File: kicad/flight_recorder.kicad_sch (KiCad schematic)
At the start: 12 parts, among them Q3 FS8205A, U1 ESP32-C3-SuperMini, U2 DW01A, U3 MCP1700x-330xxTT

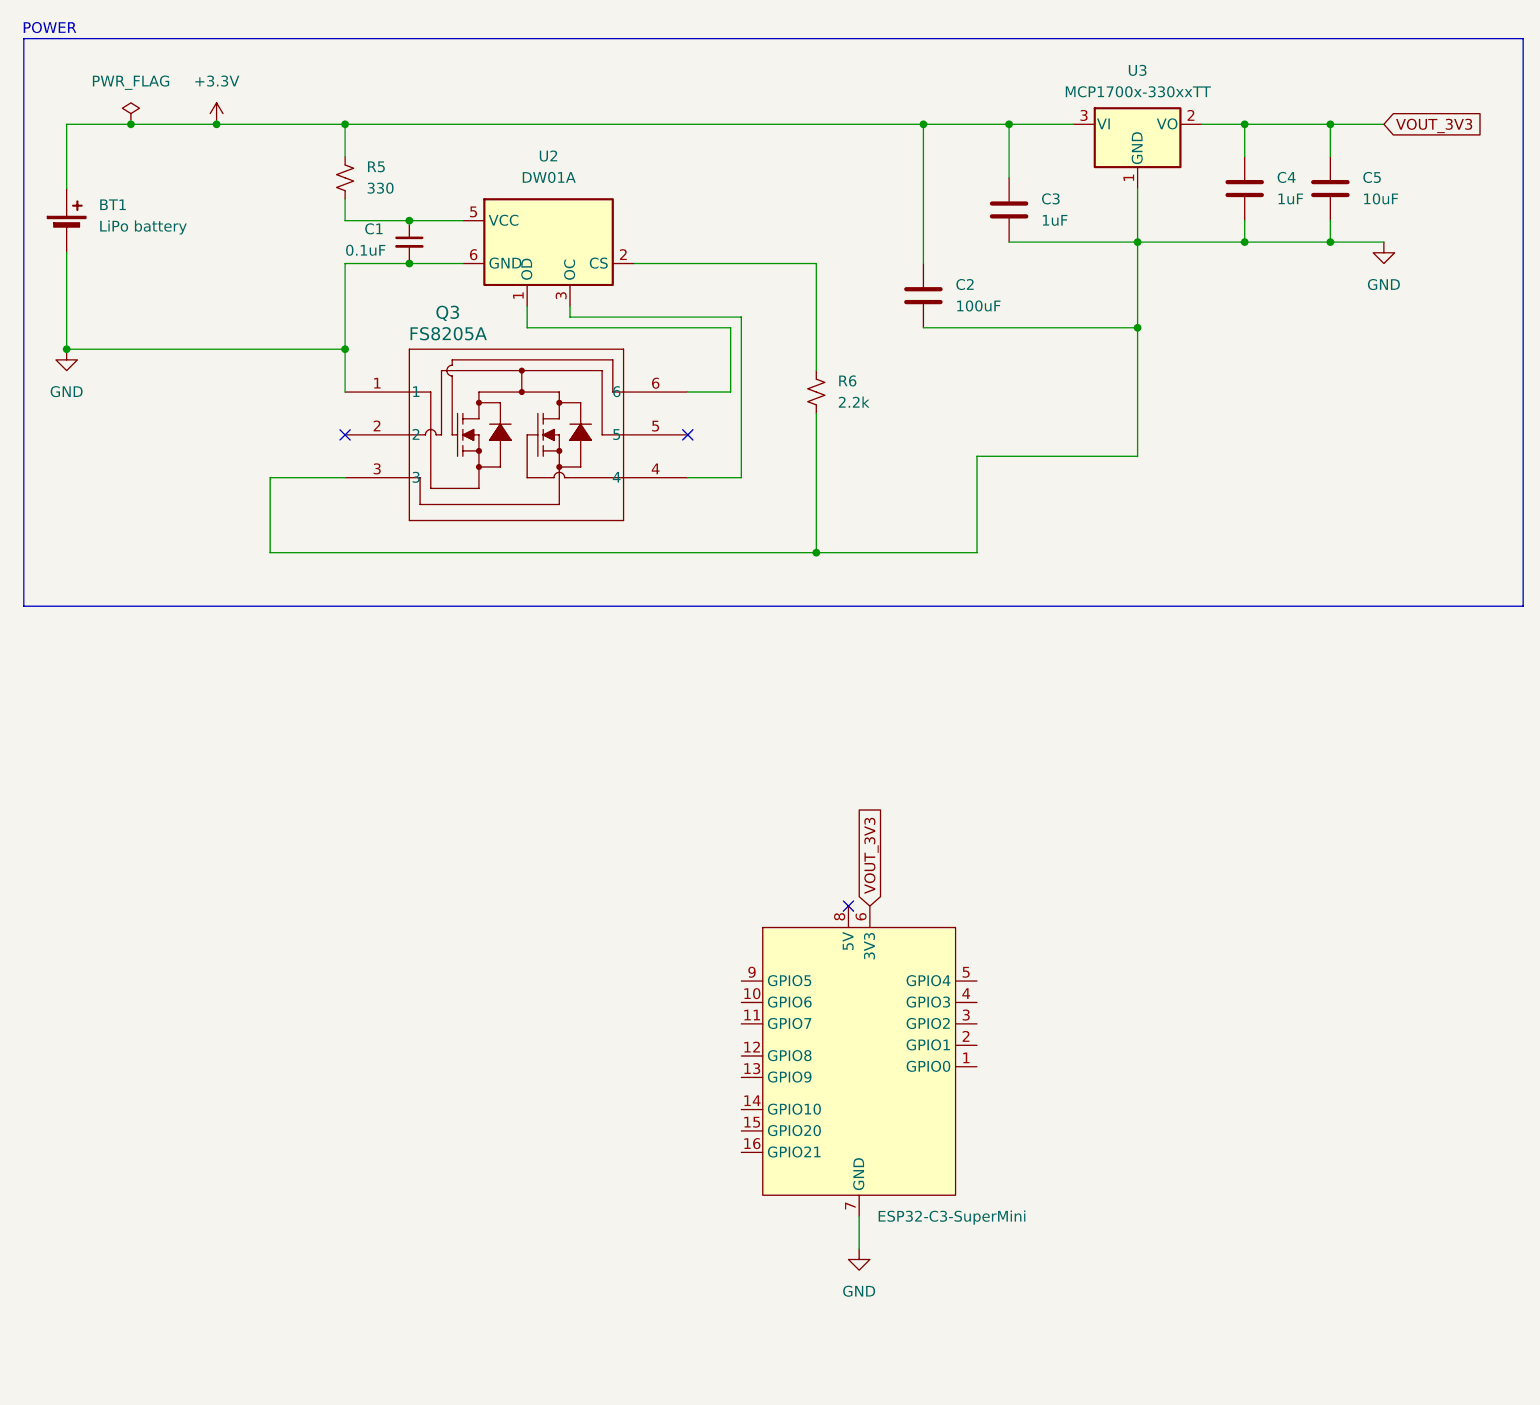
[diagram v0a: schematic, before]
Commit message: added sensors
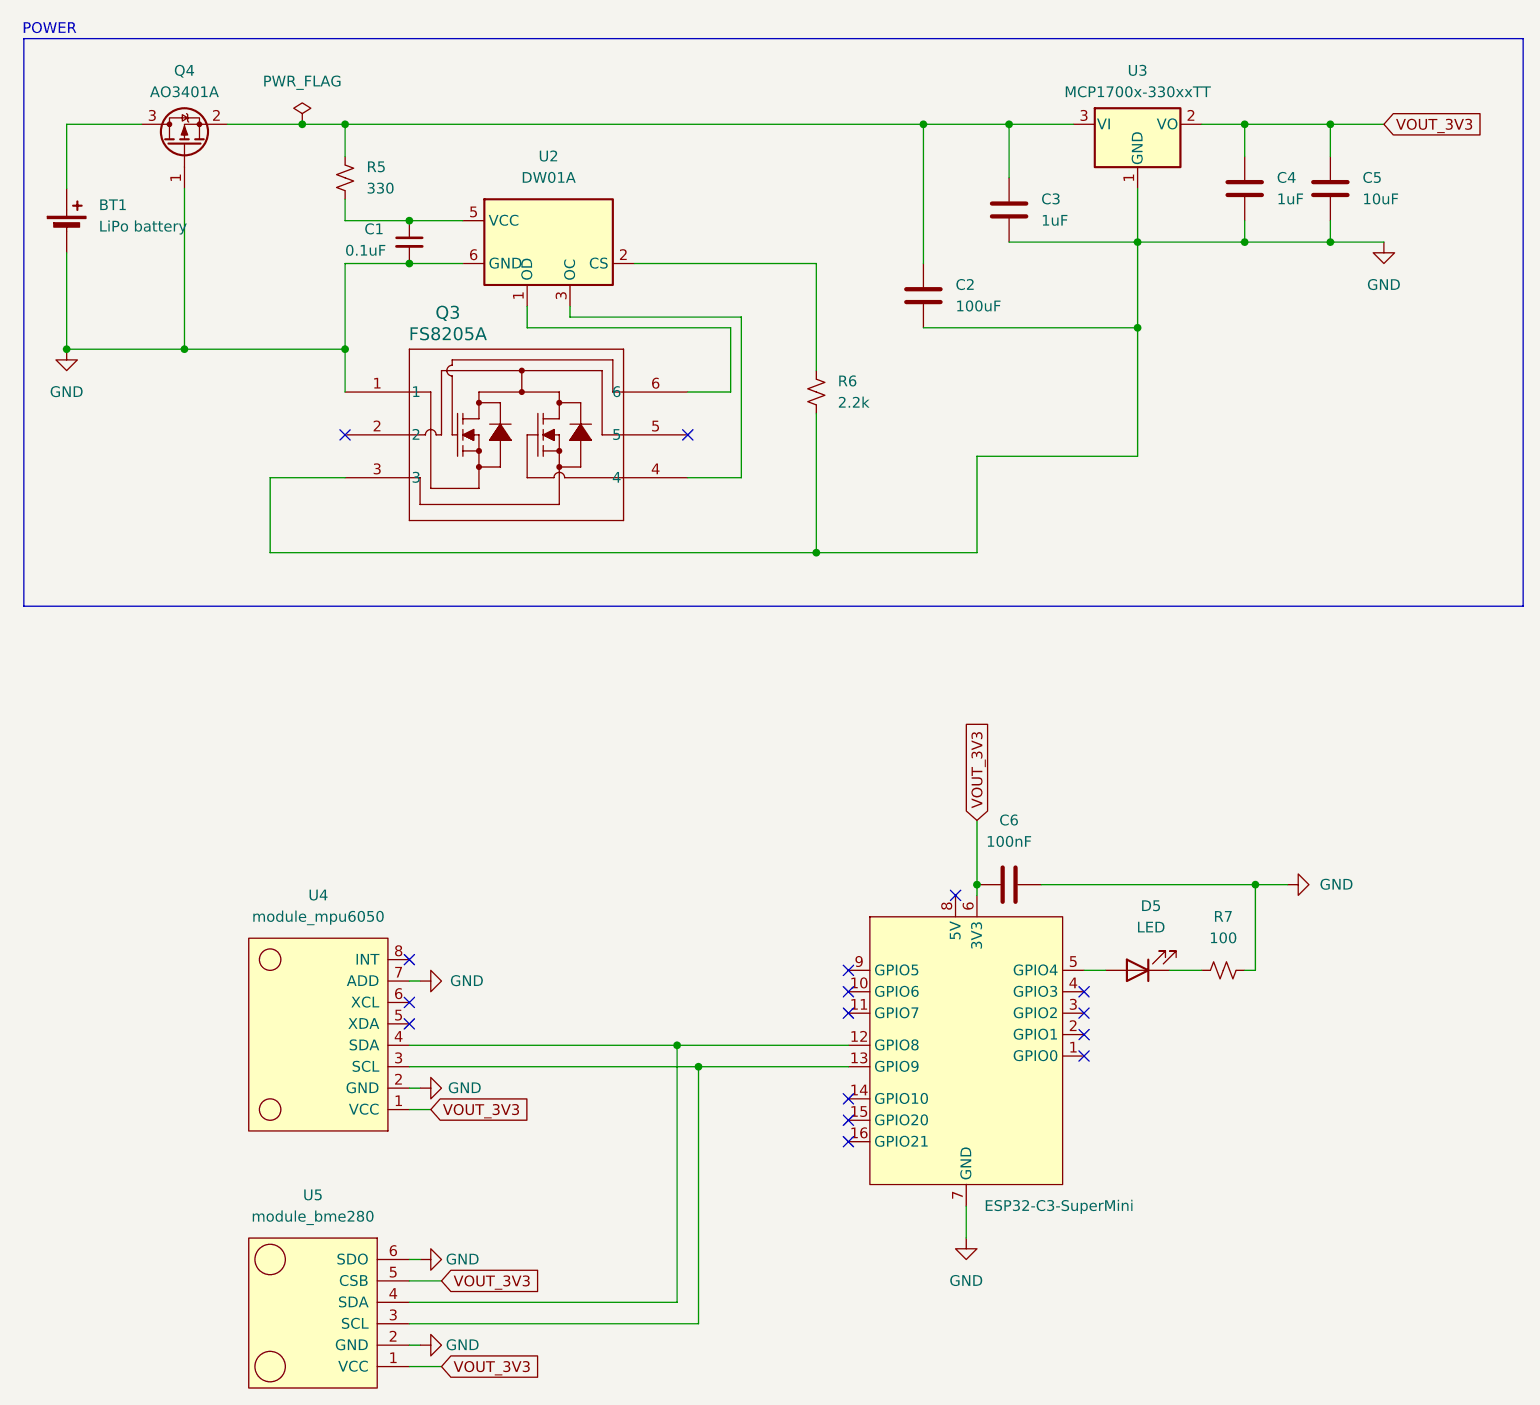
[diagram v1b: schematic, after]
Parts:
- added C6: 100nF, Capacitor_SMD:C_1206_3216Metric_Pad1.33x1.80mm_HandSolder, symbol Device:C
- added D5: LED, LED_SMD:LED_1210_3225Metric_Pad1.42x2.65mm_HandSolder, symbol Device:LED
- added Q4: AO3401A, Package_TO_SOT_SMD:SOT-23, symbol Transistor_FET:AO3401A
- added R7: 100, Resistor_SMD:R_0805_2012Metric_Pad1.20x1.40mm_HandSolder, symbol Device:R_Small_US
- added U4: module_mpu6050, usini_sensors:module_mpu6050, symbol usini_sensors:module_mpu6050
- added U5: module_bme280, usini_sensors:module_bme280, symbol usini_sensors:module_bme280
- U1: Buy (none) -> https://makerbazar.in/products/esp32-c3-supermini-iot-devel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; Buy_ALT (none) -> https://www.amazon.in/DELLZO-ESP32-C3-Development-Bluetooth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
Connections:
- net GND: now also C6.2, Q4.1 (G), R7.2, U4.2 (GND), U4.7 (ADD), U5.2 (GND), U5.6 (SDO)
- net VOUT_3V3: now also C6.1, U4.1 (VCC), U5.1 (VCC), U5.5 (CSB)
- net at U1.12 (GPIO8): now also U4.4 (SDA), U5.4 (SDA)
- net at U1.13 (GPIO9): now also U4.3 (SCL), U5.3 (SCL)
- net at U1.5 (GPIO4): now also D5.2 (A)
- net +3.3V: no longer names the net of C2.1, C3.1, R5.1, U3.3 (VI)
- net +3.3V: now also Q4.2 (S); no longer BT1.1 (+)
- new net: BT1.1 (+), Q4.3 (D)
- new net: D5.1 (K), R7.1
- no-connect marks 3 -> 16
